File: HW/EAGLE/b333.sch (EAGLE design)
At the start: 211 parts, among them Q1 2N4126, Q2 2N4126, Q5 NMOSD, X1 USB MICRO

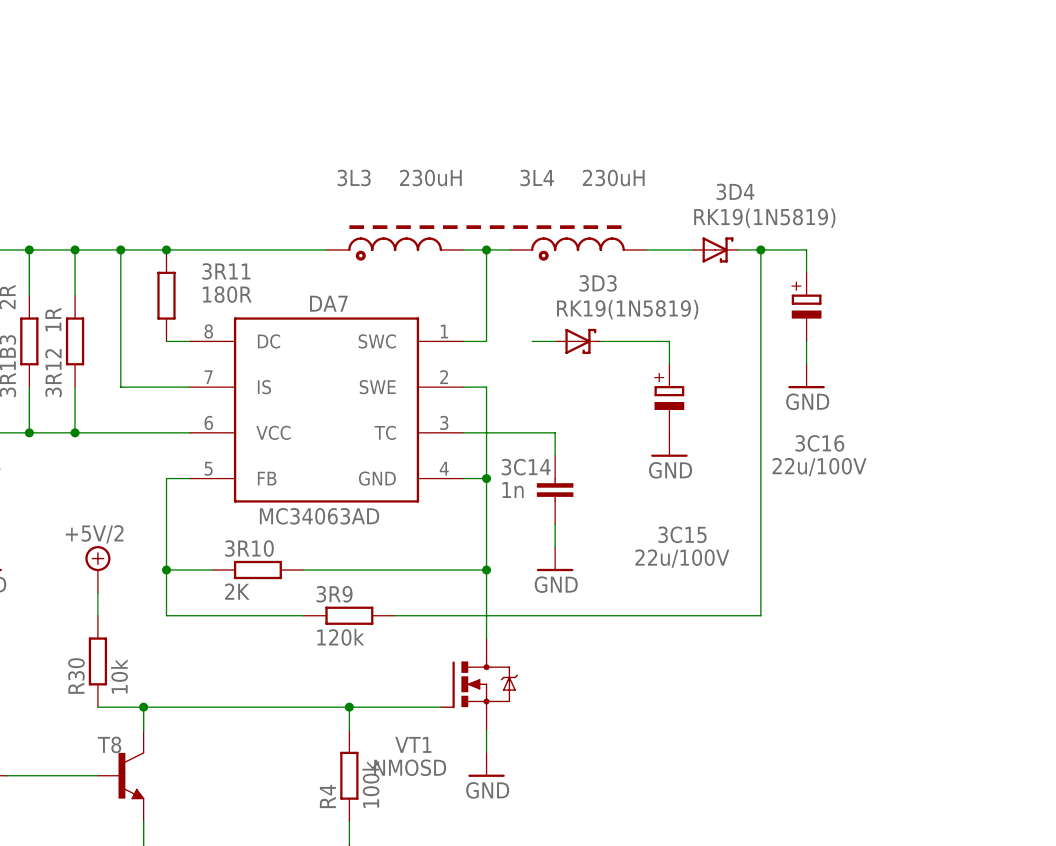
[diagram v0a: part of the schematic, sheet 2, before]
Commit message: sch
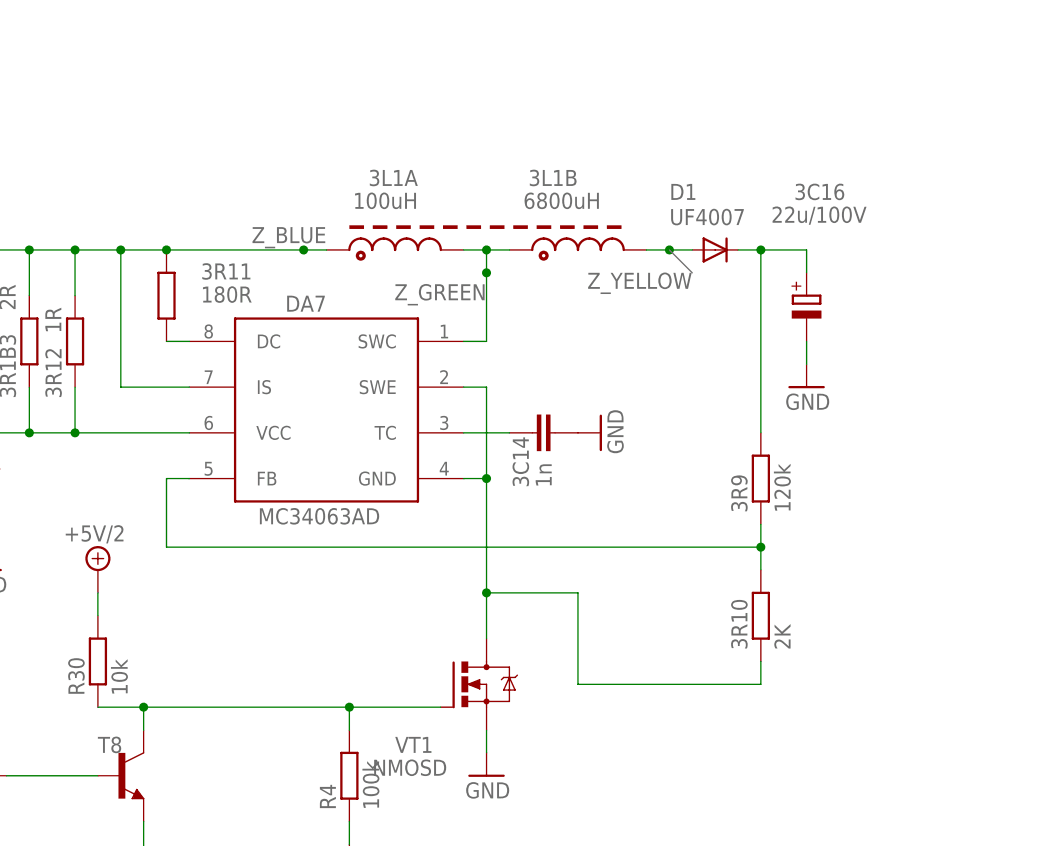
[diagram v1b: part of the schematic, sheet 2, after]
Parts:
- removed 3C15: 22u/100V, resistor:CPOL-EUE2.5-6
- removed 3D3, 3D4: RK19(1N5819), diode:SCHOTTKY-DIODESMD
- added D1: UF4007, diode:1N4004
- 3L1A: value 230uH -> 100uH
- 3L1B: value 230uH -> 6800uH
- renumbered 3L3 to 3L1A, 3L4 to 3L1B
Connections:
- net N$24 renamed Z_GREEN
- net N$56 renamed Z_BLUE
- removed net N$45: 3D3.A
- removed net N$57: 3R10.2, DA7.GND, DA7.SWE, VT1.D
- removed net N$73: 3D4.A, 3L1B.2
- new net Z_YELLOW: 3L1B.2, D1.A
- net GND: no longer 3C15.-
- net N$12: now also 3R10.1, DA7.GND, DA7.SWE, VT1.D; no longer 3C15.+, 3D3.C
- net N$25: now also 3R10.2; no longer 3R10.1
- net N$94: now also D1.C; no longer 3D4.C
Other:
- moved on the sheet: 3C14, 3R10, 3R9

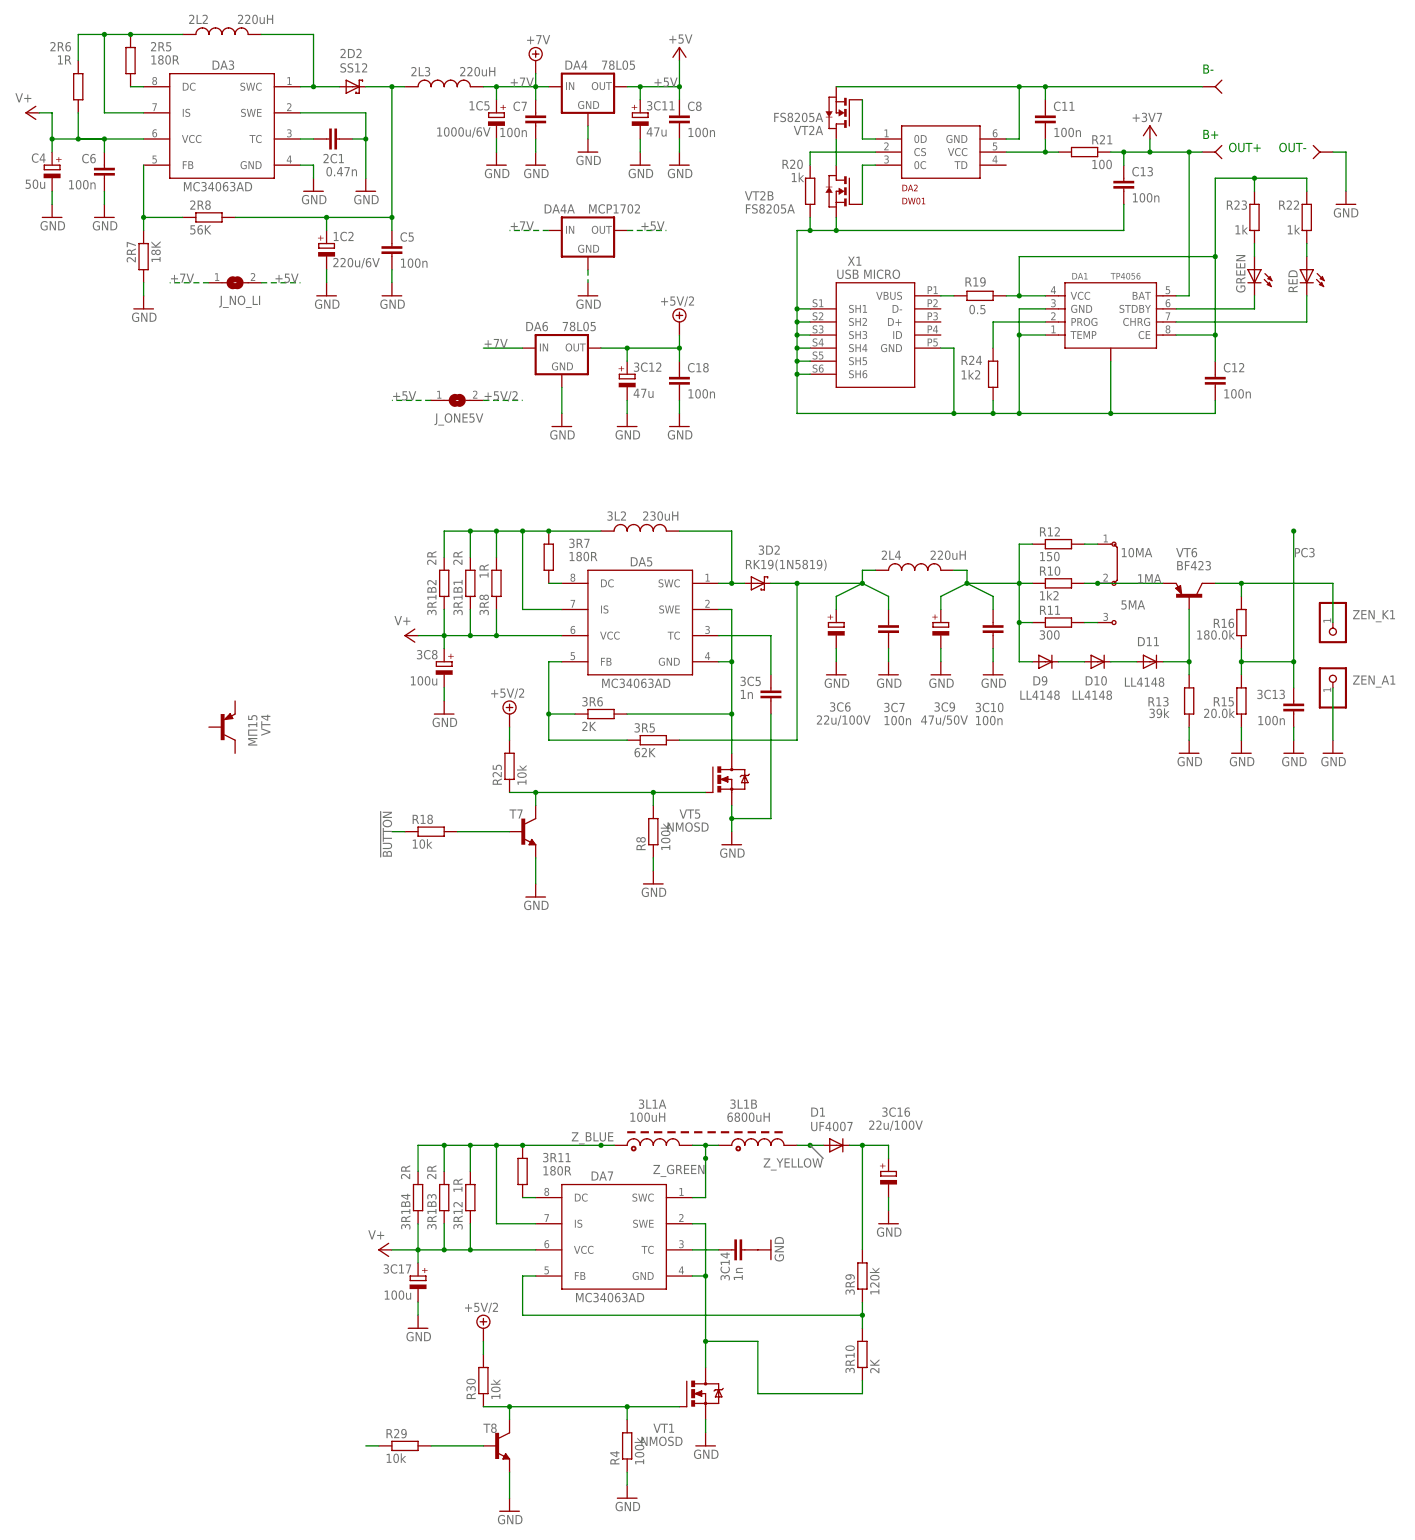
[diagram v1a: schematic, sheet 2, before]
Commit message: .
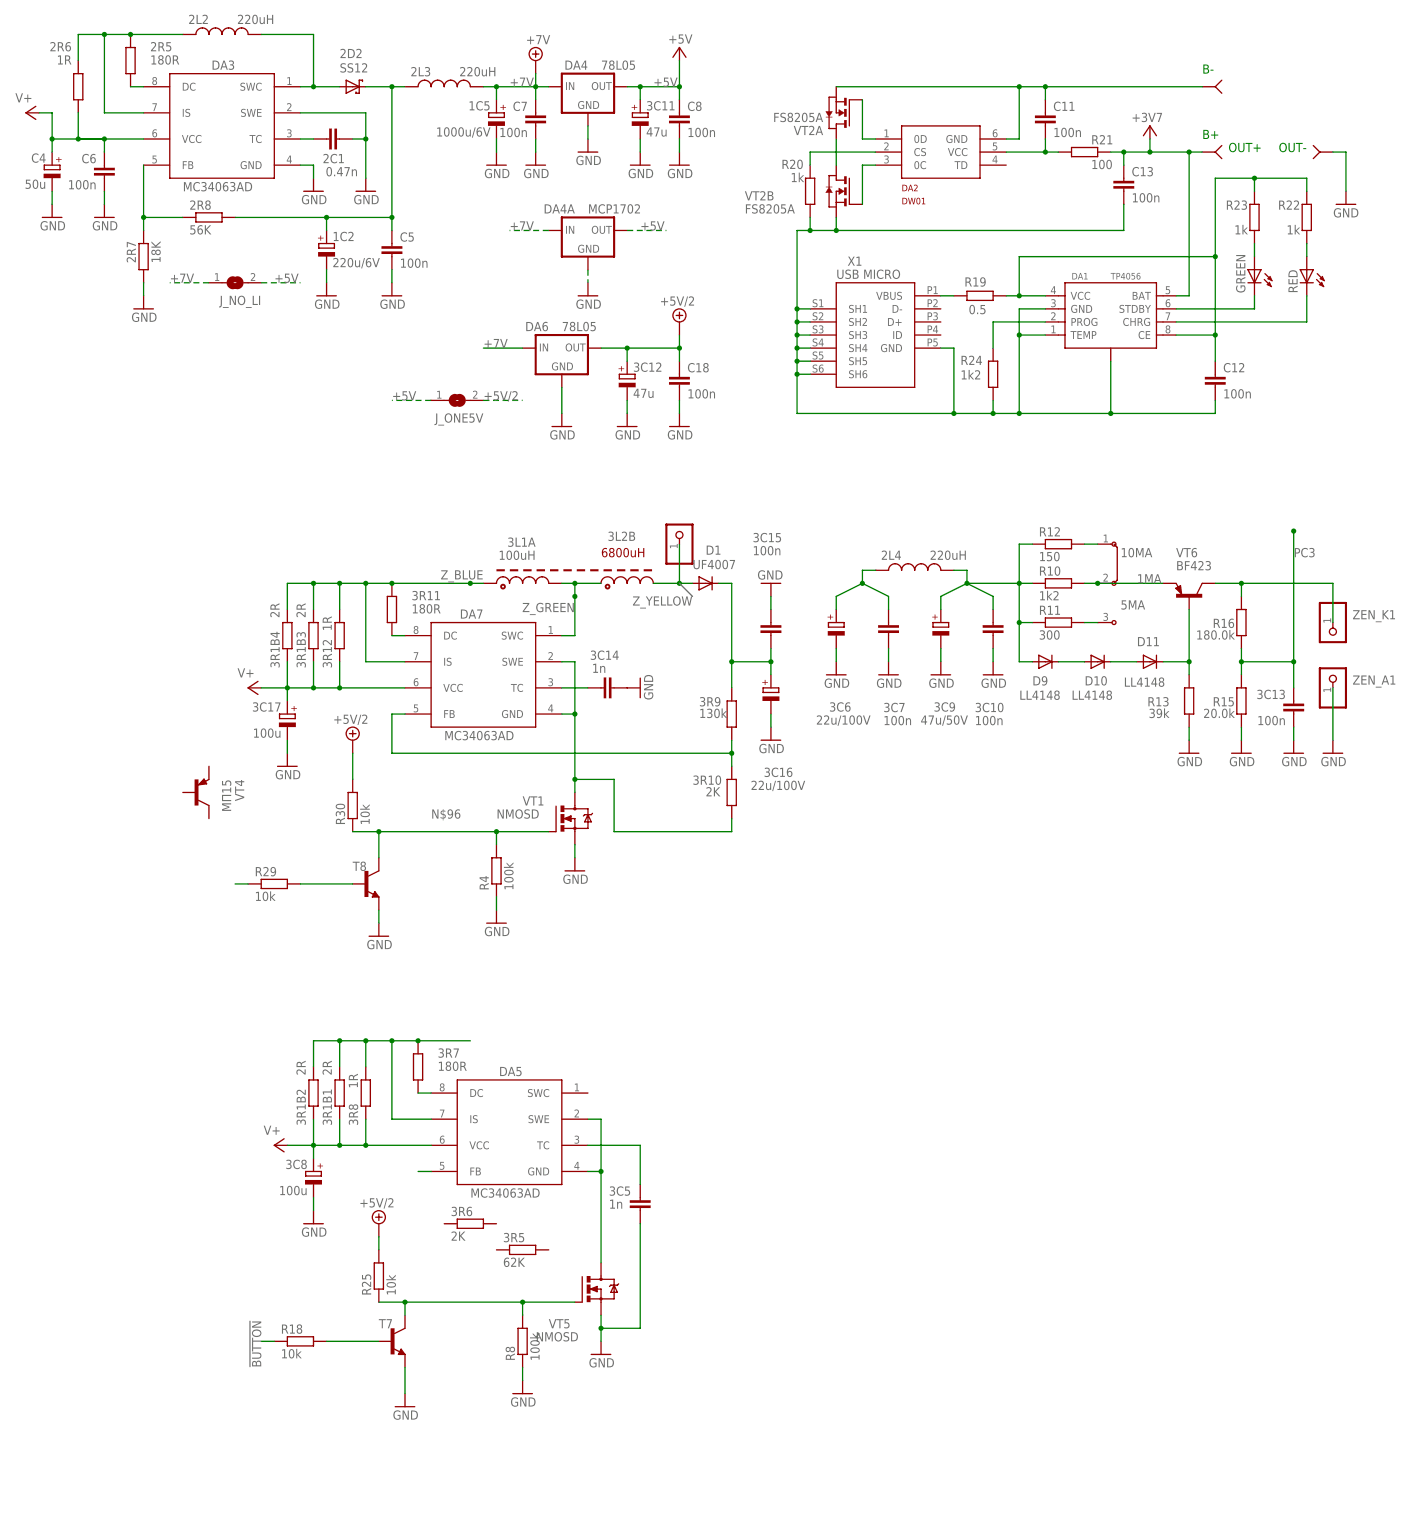
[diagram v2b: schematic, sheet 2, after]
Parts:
- removed 3D2: RK19(1N5819), diode:SCHOTTKY-DIODESMD
- removed 3L1B: 6800uH, rcl:L-US6000-XXX-RC
- removed 3L2: 230uH, rcl:L-US6000-XXX-RC
- added 3C15: 100n, resistor:C-EU025-025X050
- added 3L2B: (no value), pinhead:PINHD-1X1
- 3C16: device resistor:CPOL-EUE2.5-6 -> resistor:CPOL-EUE5-8.5
- 3R9: value 120k -> 130k
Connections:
- removed net N$26: 3D2.A, 3L2.2, DA5.SWC
- removed net N$92: 2L4.1, 3C6.+, 3C7.1, 3D2.C, 3R5.2
- removed net N$94: 3C16.+, 3R9.2, D1.C
- new net N$24: 3C15.2, 3C16.+, 3R9.2, D1.C
- new net N$45: 2L4.1, 3C6.+, 3C7.1
- net GND: now also 3C15.1
- net N$51: no longer 3R5.1, 3R6.1
- net N$54: no longer 3L2.1
- net N$58: no longer 3R6.2
- net Z_GREEN: no longer 3L1B.1
- net Z_YELLOW: now also 3L2B.1; no longer 3L1B.2
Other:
- note added: "+20V"
- note added: "10mm"
- note added: "13-14mm"
- note added: "2k"
- note added: "30k"
- note added: "34R1"
- note added: "34R2"
- note added: "5mm"
- note added: "6800uH"
- note added: "7mm"
- note added: "I 49w 0.32mm > 105uH II 400w 0.15mm > 6.8mH"
- note added: "SS16"
- moved on the sheet: 3C14, 3C16, 3C17, 3C5, 3C8, 3L1A, 3R10, 3R11, 3R12, 3R1B1, 3R1B2, 3R1B3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

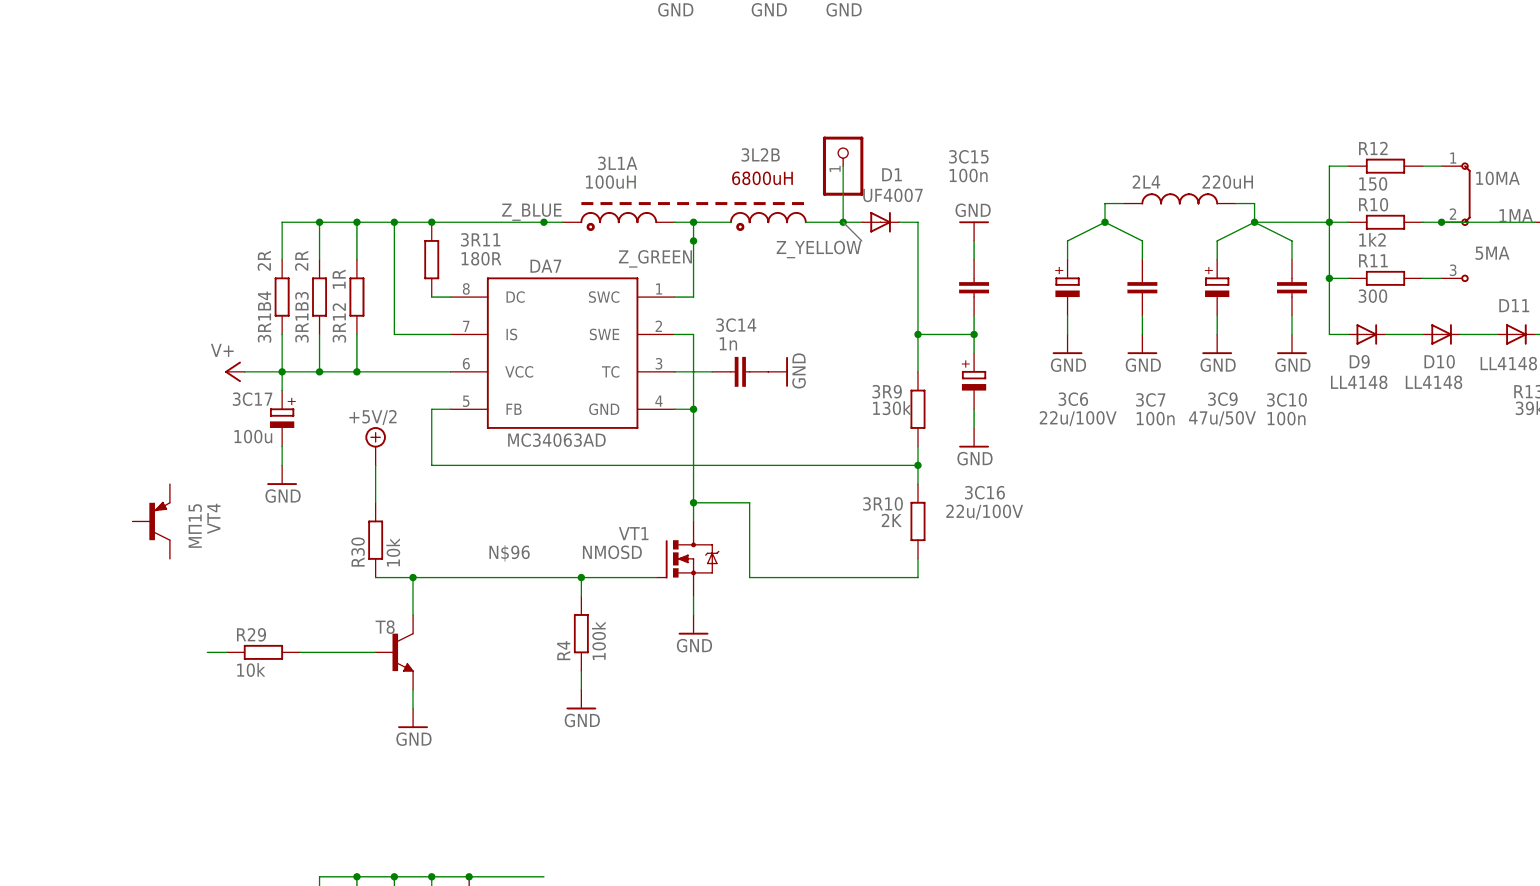
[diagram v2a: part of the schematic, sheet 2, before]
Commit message: .
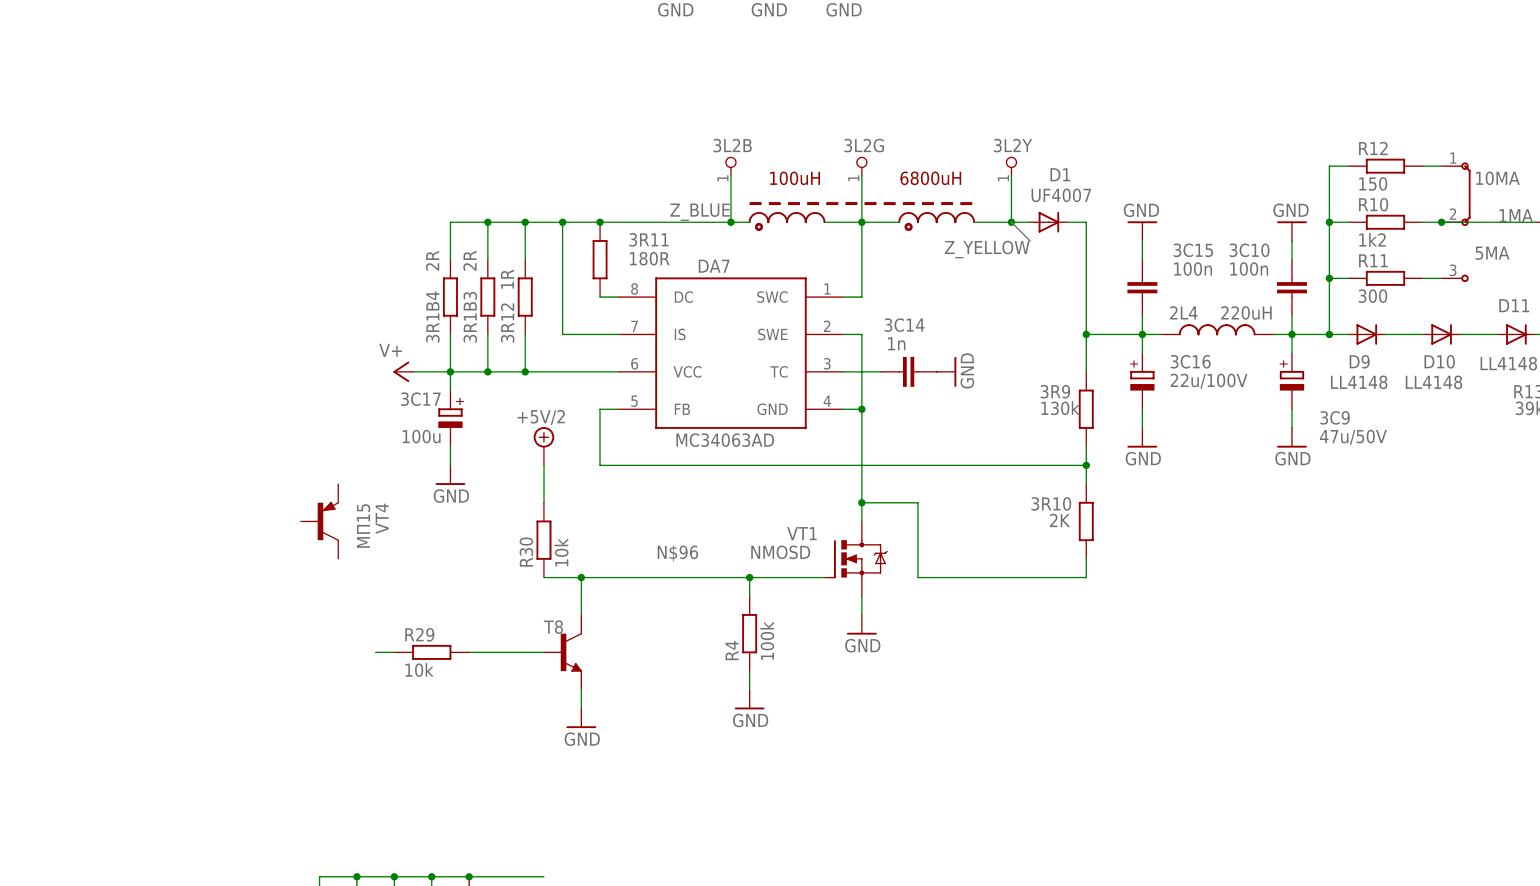
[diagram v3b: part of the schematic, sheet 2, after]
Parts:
- removed 3C6: 22u/100V, resistor:CPOL-EUE2.5-6
- removed 3C7: 100n, resistor:C-EUC0805K
- removed 3L1A: 100uH, rcl:L-US6000-XXX-RC
- added 3L2G, 3L2Y: (no value), b333:PINHD-1X1
- added L: L, b333:L
- 3C16: device resistor:CPOL-EUE5-8.5 -> resistor:CPOL-EUTT5D9L
- 3L2B: device pinhead:PINHD-1X1 -> b333:PINHD-1X1
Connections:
- removed net N$45: 2L4.1, 3C6.+, 3C7.1
- net +40V: now also 3C10.2; no longer 3C10.1
- net GND: now also 3C10.1; no longer 3C10.2, 3C6.-, 3C7.2
- net N$24: now also 2L4.1
- net Z_BLUE: now also 3L2B.1; no longer 3L1A.1
- net Z_GREEN: now also 3L2G.1; no longer 3L1A.2
- net Z_YELLOW: now also 3L2Y.1; no longer 3L2B.1
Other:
- note added: "100uH"
- note removed: "10mm"
- note removed: "13-14mm"
- note removed: "5mm"
- note removed: "7mm"
- moved on the sheet: 2L4, 3C14, 3C15, 3C16, 3C17, 3C9, 3R10, 3R11, 3R12, 3R1B3, 3R1B4, 3R9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
